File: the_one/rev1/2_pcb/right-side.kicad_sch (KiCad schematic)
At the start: 39 parts, among them SW20 KeySwitch, SW21 KeySwitch, SW22 KeySwitch, SW23 KeySwitch, SW24 KeySwitch, SW25 KeySwitch, SW26 KeySwitch, SW27 KeySwitch, SW28 KeySwitch, SW29 KeySwitch, SW30 KeySwitch, SW31 KeySwitch, SW32 KeySwitch, SW33 KeySwitch, SW34 KeySwitch, SW35 KeySwitch, SW36 KeySwitch, SW37 KeySwitch, SW38 KeySwitch, U2 Pico

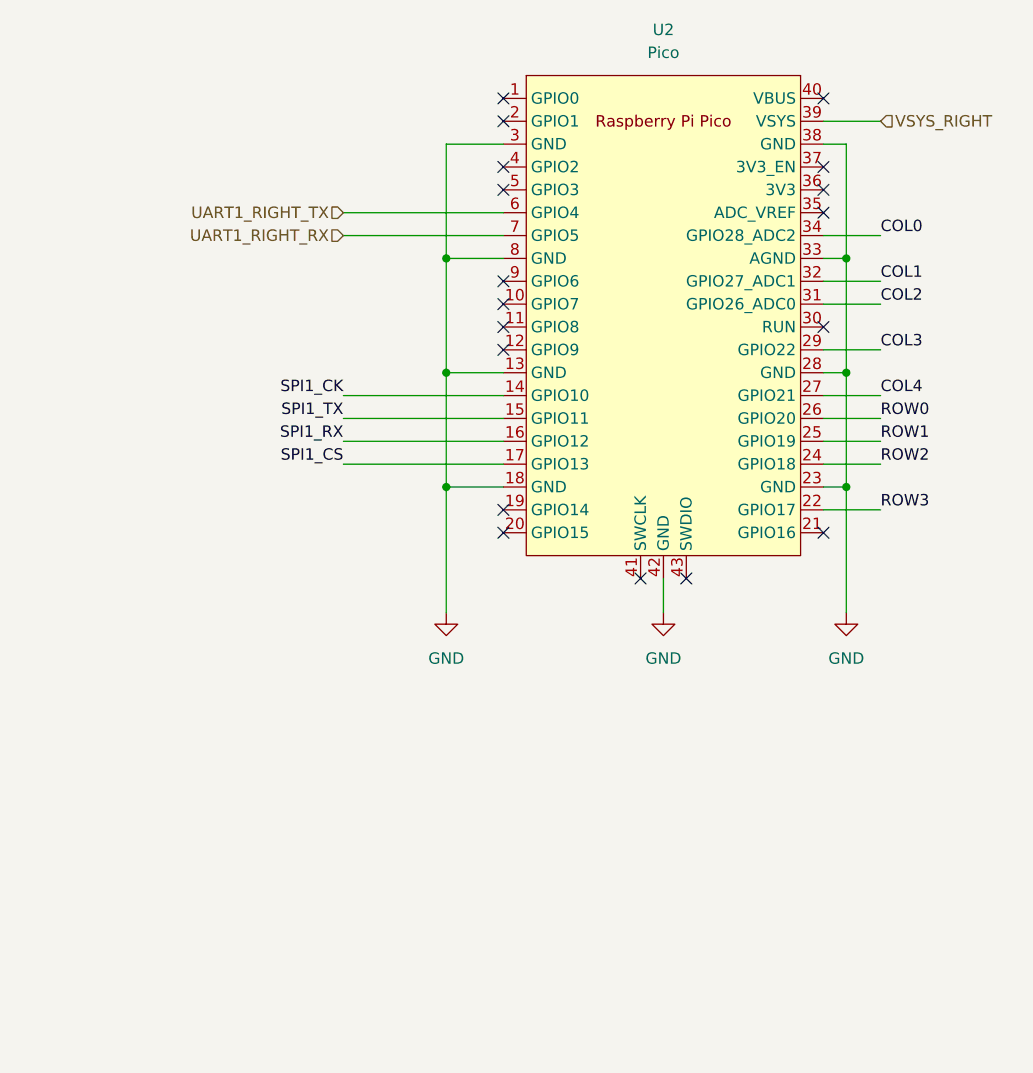
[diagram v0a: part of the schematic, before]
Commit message: update KiCAD schematcis
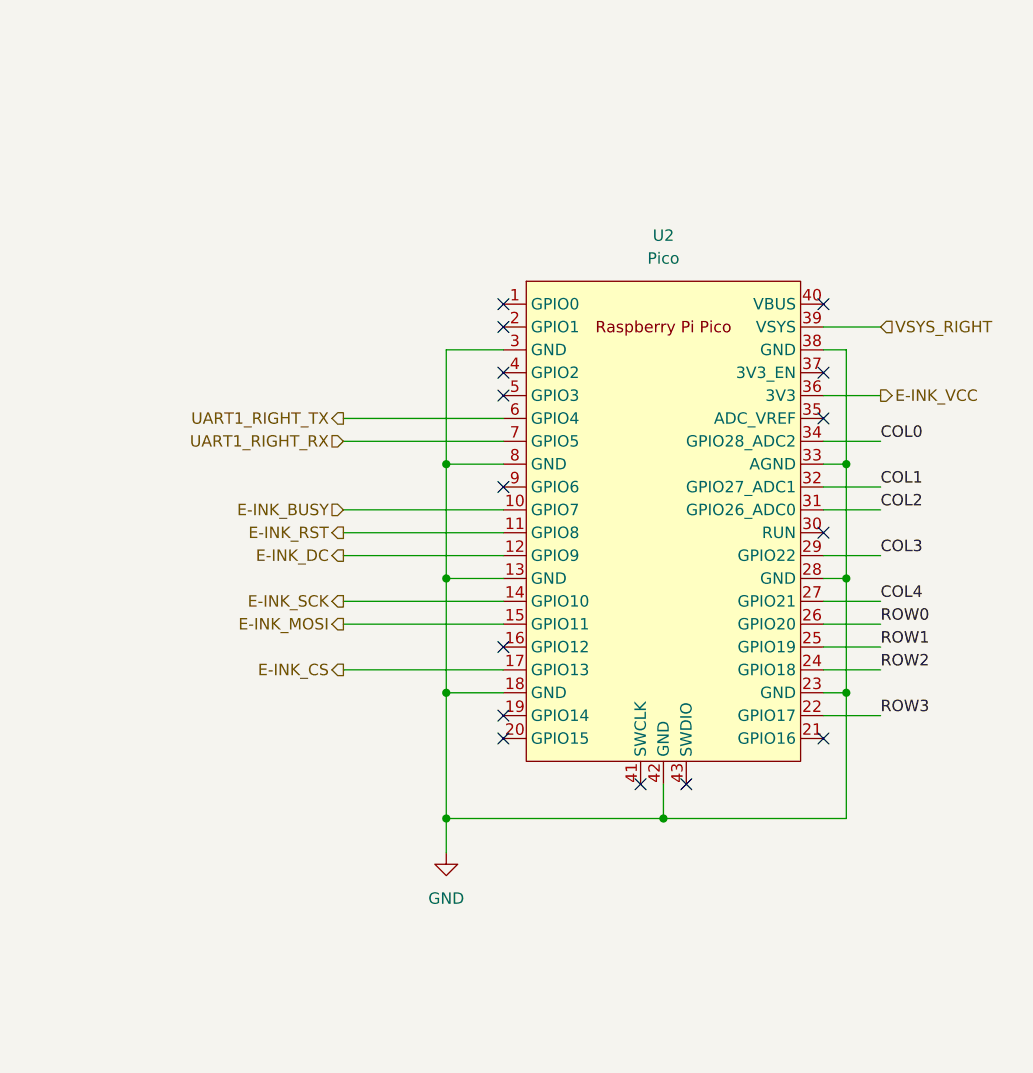
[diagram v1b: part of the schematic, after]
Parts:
- U2: footprint RPi_Pico:RPi_Pico_SMD_TH -> MCU_RaspberryPi_and_Boards:RPi_Pico_SMD_TH
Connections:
- net E-INK_BUSY: now reaches U2.10 (GPIO7)
- net E-INK_RST: now reaches U2.11 (GPIO8)
- net E-INK_DC: now reaches U2.12 (GPIO9)
- net E-INK_VCC: now reaches U2.36 (3V3)
- net SPI1_CK renamed E-INK_SCK
- net SPI1_CS renamed E-INK_CS
- net SPI1_RX: no longer names the net of U2.16 (GPIO12)
- net SPI1_TX renamed E-INK_MOSI
- no-connect marks 18 -> 15
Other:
- moved on the sheet: U2
